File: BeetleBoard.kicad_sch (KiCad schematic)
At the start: 26 parts, among them J16 ESC G, J17 ESC H, J18 ELRS Reciever, J2 ESC A, J3 ESC B, J4 ESC C, J5 ESC D, J6 ESC E, J7 ESC F, U1 XIAO-ESP32-C6-SMD

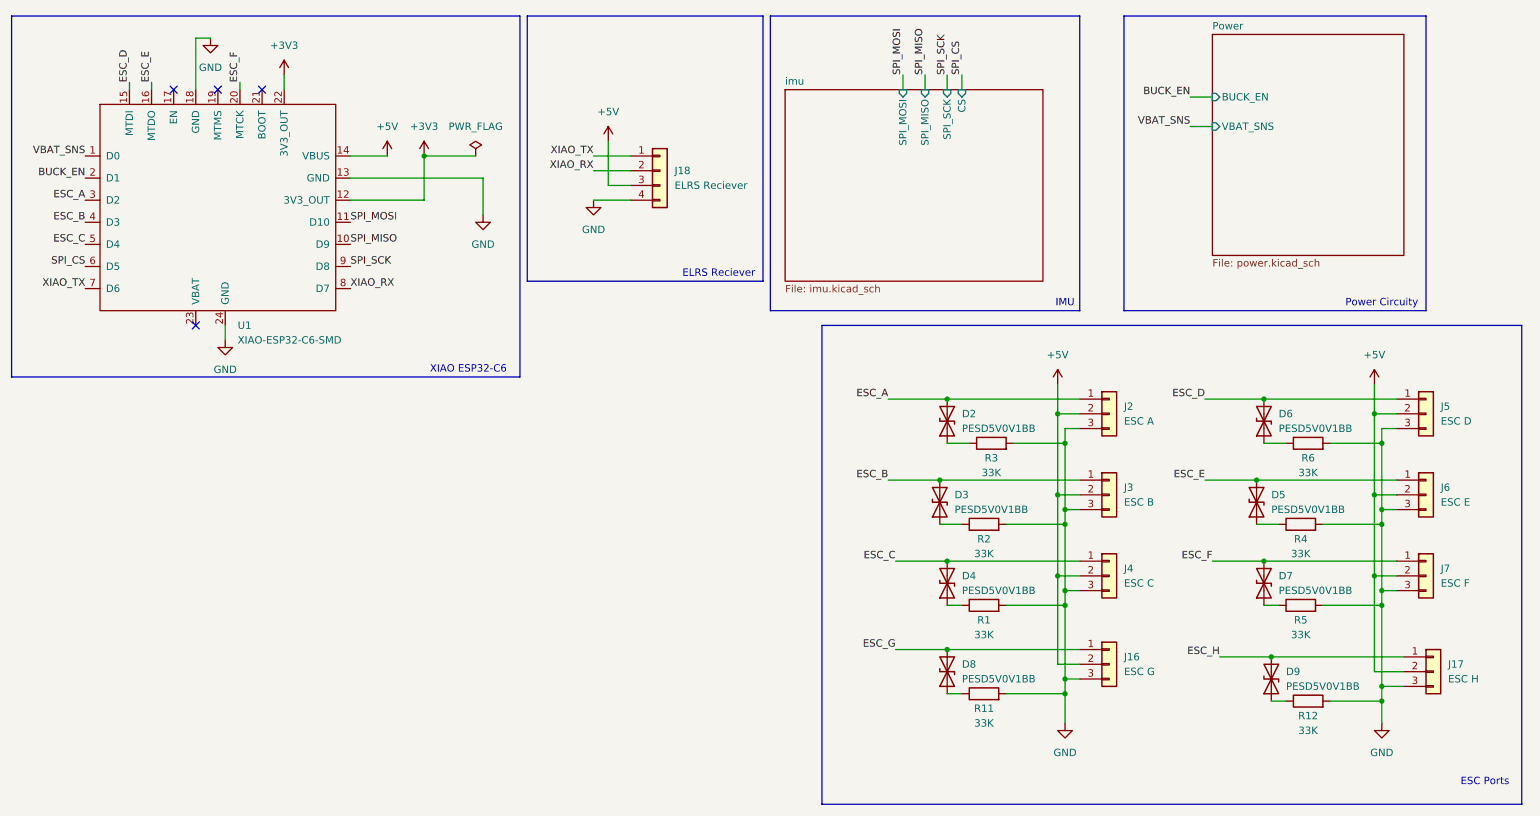
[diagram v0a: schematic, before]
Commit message: clean up schematics and start pcb
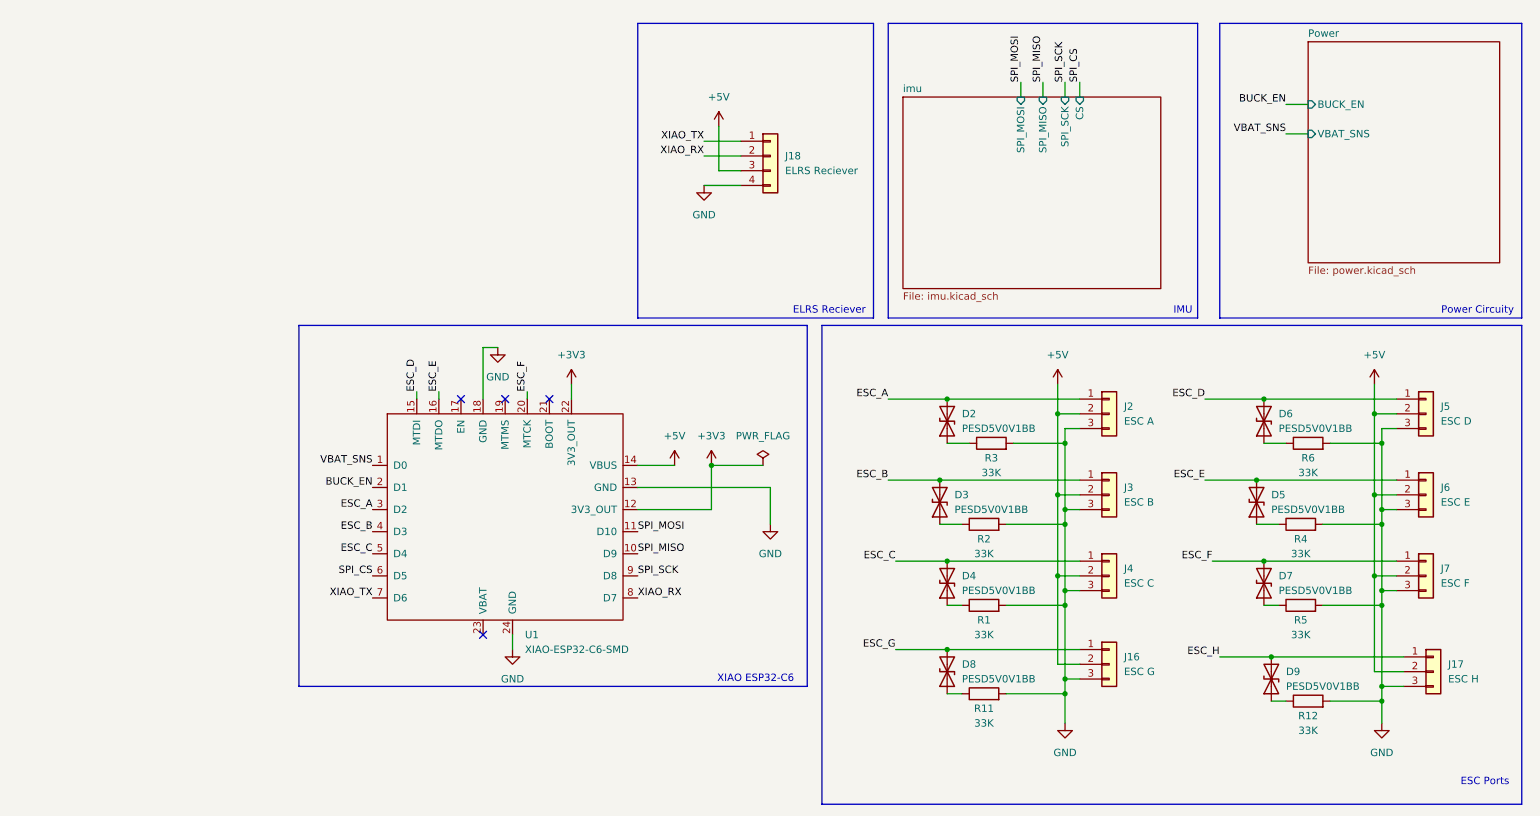
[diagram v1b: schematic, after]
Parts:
- D2, D3, D4, D5, D6, D7, D8, D9: footprint (none) -> Diode_SMD:D_SOD-323
- J16, J17, J2, J3, J4, J5, J6, J7: footprint (none) -> Connector_PinHeader_2.54mm:PinHeader_1x03_P2.54mm_Vertical
- J18: footprint (none) -> footprints:BetaFPV_ELRS_Lite
- R1, R11, R12, R2, R3, R4, R5, R6: footprint (none) -> Resistor_SMD:R_0805_2012Metric_Pad1.20x1.40mm_HandSolder
- U1: footprint Seeed_Studio_XIAO_Series:XIAO-ESP32-C6-SMD -> Seeed Studio XIAO Series Library:XIAO-ESP32-C6-SMD
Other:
- moved on the sheet: J18, U1
